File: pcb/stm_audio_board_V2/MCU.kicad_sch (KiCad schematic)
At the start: 9 parts, among them SW1 SW_SPST, U3 STM32H747IGTx, Y2 X1E0000210132

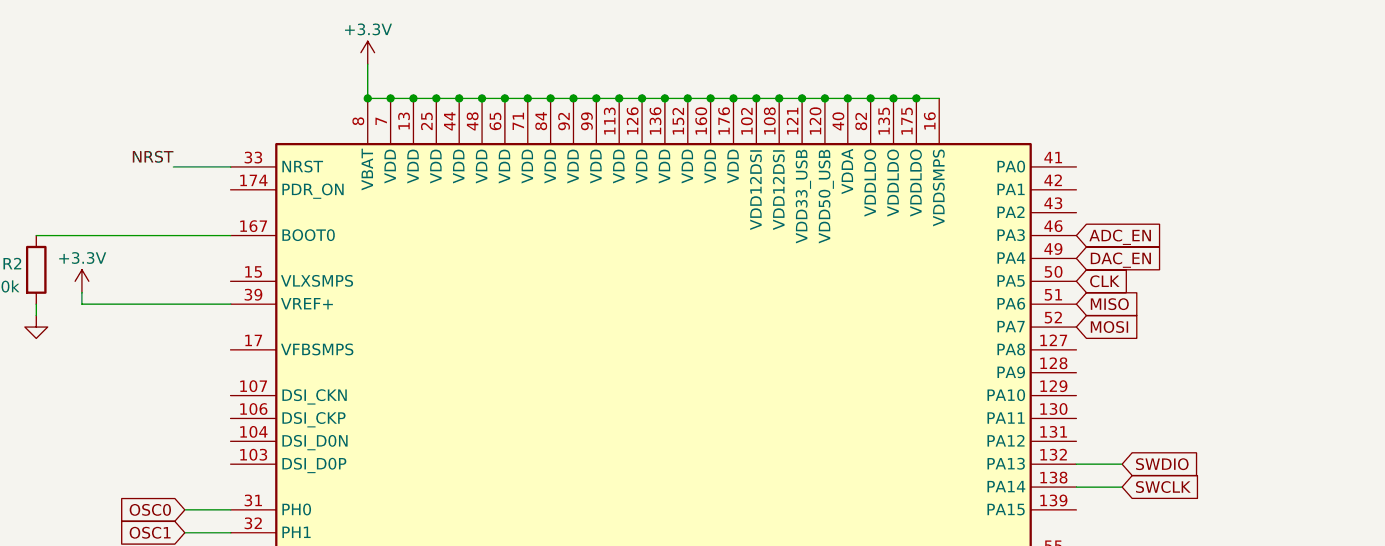
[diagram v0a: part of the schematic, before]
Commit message: smps setup is used
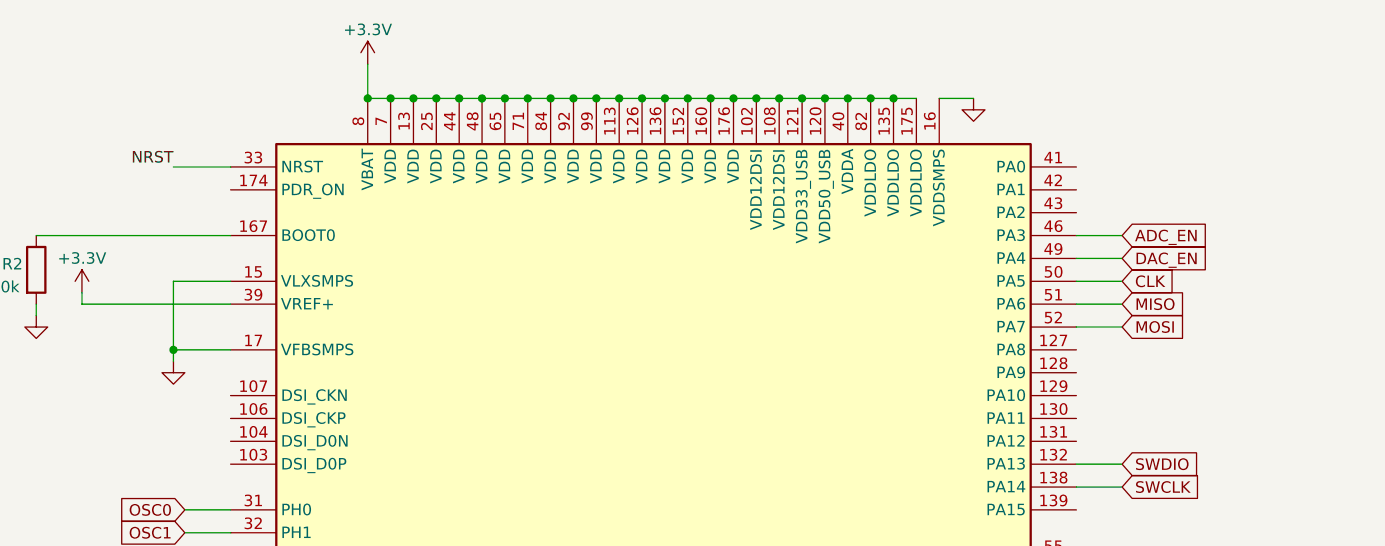
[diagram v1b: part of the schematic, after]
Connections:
- net +3.3V: no longer U3.16 (VDDSMPS)
- net GND: now also U3.15 (VLXSMPS), U3.16 (VDDSMPS), U3.17 (VFBSMPS)
